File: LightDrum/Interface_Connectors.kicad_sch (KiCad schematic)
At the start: 6 parts, among them J6 0525593652, J7 0541323662, J8 PWR-CONN

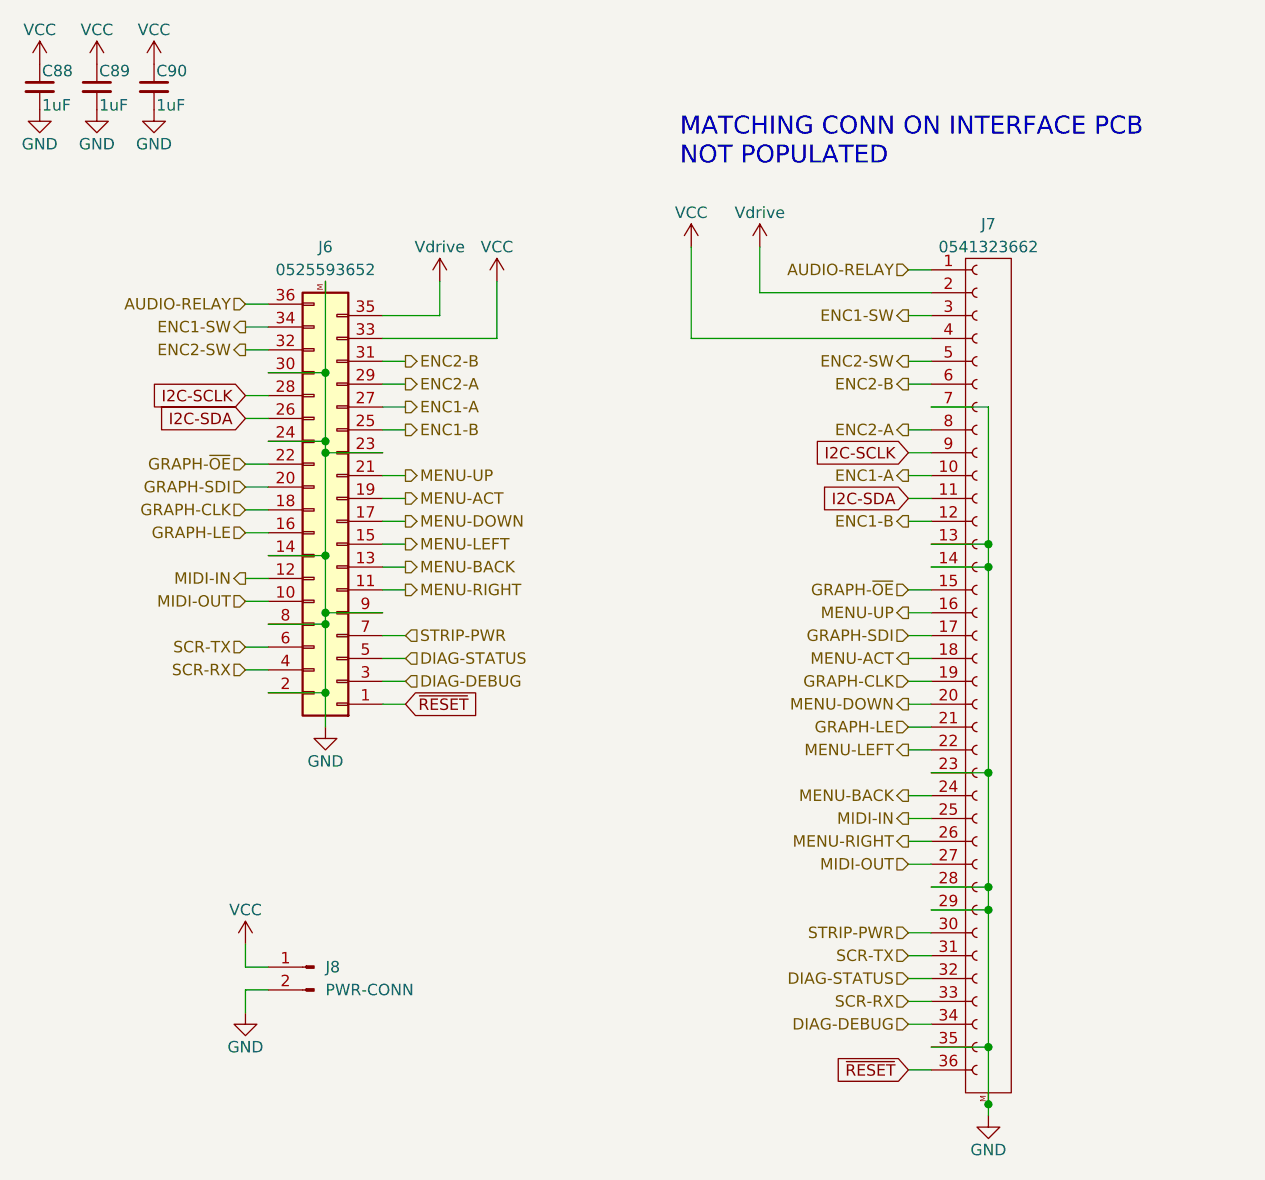
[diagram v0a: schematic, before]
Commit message: First pass over schematic (WIP)
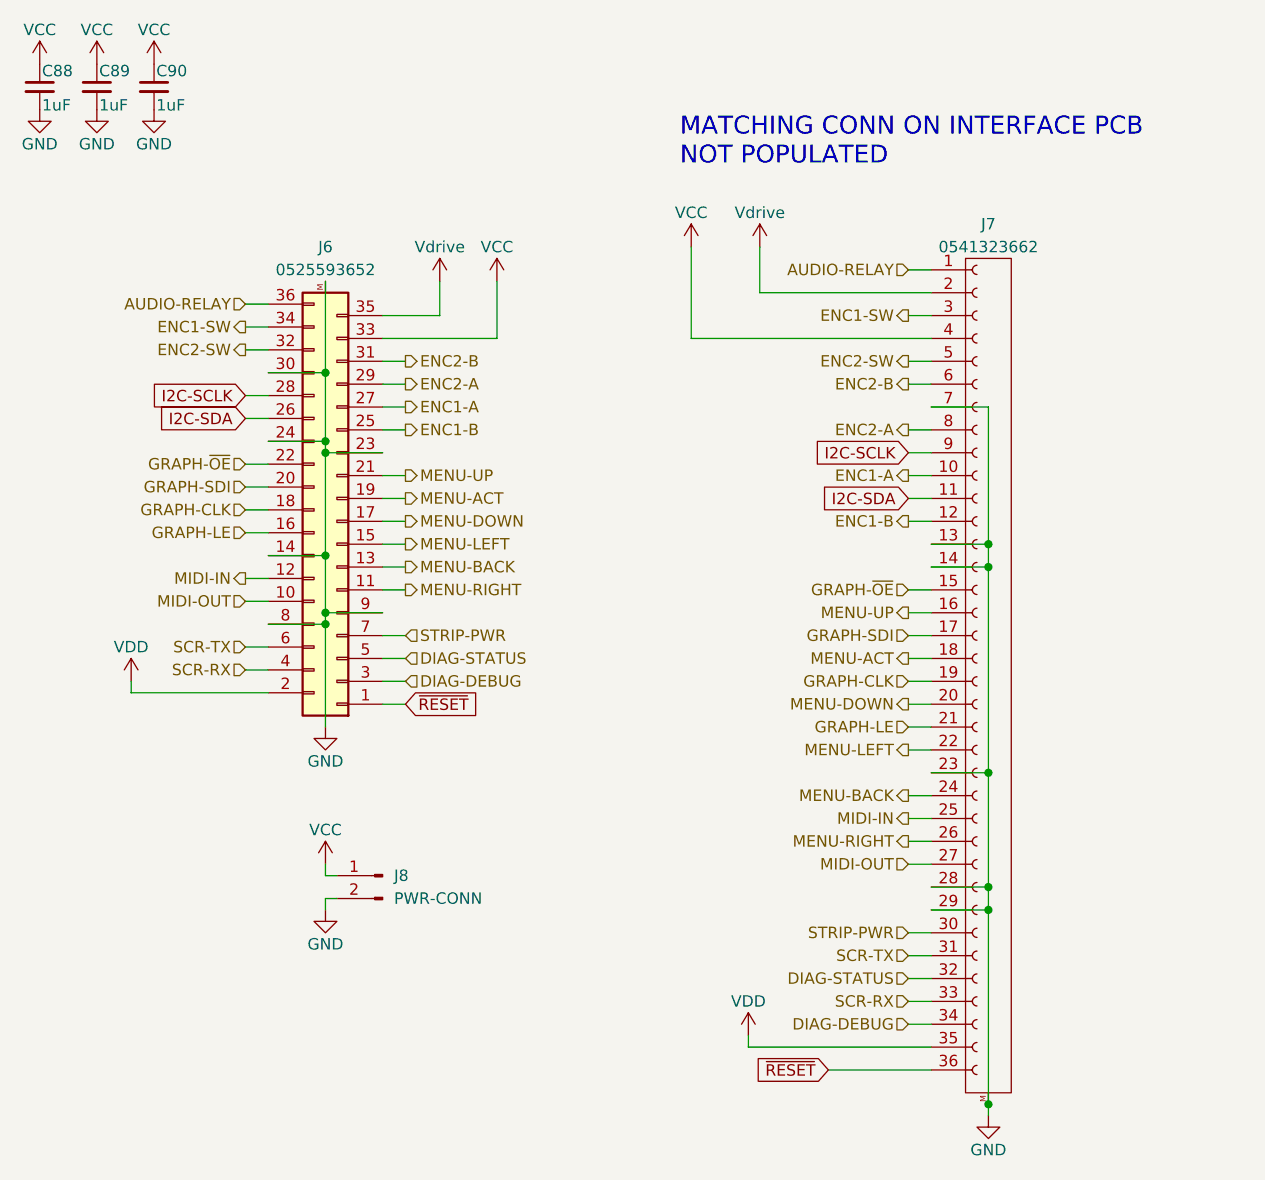
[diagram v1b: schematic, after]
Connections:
- net GND: no longer J6.2 (Pin_2), J7.35 (Pin_35)
- new net VDD: J6.2 (Pin_2), J7.35 (Pin_35)
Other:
- moved on the sheet: J8
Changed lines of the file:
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@@
   (title_block
     (title "LightDrum")
-    (rev "REV7")
+    (rev "REV8")
     (company "Daxxn Industries")
   )
-  (junction (at 50.8 90.17) (diameter 0) (color 0 0 0 0)
-  )
   (junction (at 124.46 76.2) (diameter 0) (color 0 0 0 0)
   )
@@
   (junction (at 50.8 62.23) (diameter 0) (color 0 0 0 0)
   )
-  (junction (at 124.46 129.54) (diameter 0) (color 0 0 0 0)
-  )
   (junction (at 50.8 54.61) (diameter 0) (color 0 0 0 0)
   )
@@
     (stroke (width 0) (type default) (color 0 0 0 0))
   )
-  (wire (pts (xy 44.45 120.65) (xy 41.91 120.65))
+  (wire (pts (xy 52.07 110.49) (xy 50.8 110.49))
     (stroke (width 0) (type default) (color 0 0 0 0))
   )
@@
     (stroke (width 0) (type default) (color 0 0 0 0))
   )
-  (wire (pts (xy 124.46 114.3) (xy 124.46 129.54))
-    (stroke (width 0) (type default) (color 0 0 0 0))
-  )
-  (wire (pts (xy 50.8 90.17) (xy 50.8 93.98))
+  (wire (pts (xy 124.46 114.3) (xy 124.46 135.89))
     (stroke (width 0) (type default) (color 0 0 0 0))
   )
@@
     (stroke (width 0) (type default) (color 0 0 0 0))
   )
-  (wire (pts (xy 115.57 132.08) (xy 118.11 132.08))
+  (wire (pts (xy 106.68 132.08) (xy 118.11 132.08))
     (stroke (width 0) (type default) (color 0 0 0 0))
   )
@@
     (stroke (width 0) (type default) (color 0 0 0 0))
   )
+  (wire (pts (xy 29.21 88.9) (xy 29.21 90.17))
+    (stroke (width 0) (type default) (color 0 0 0 0))
+  )
   (wire (pts (xy 91.44 40.64) (xy 91.44 50.8))
     (stroke (width 0) (type default) (color 0 0 0 0))
@@
     (stroke (width 0) (type default) (color 0 0 0 0))
   )
-  (wire (pts (xy 44.45 90.17) (xy 50.8 90.17))
-    (stroke (width 0) (type default) (color 0 0 0 0))
-  )
   (wire (pts (xy 69.85 50.8) (xy 57.15 50.8))
     (stroke (width 0) (type default) (color 0 0 0 0))
@@
     (stroke (width 0) (type default) (color 0 0 0 0))
   )
+  (wire (pts (xy 29.21 90.17) (xy 44.45 90.17))
+    (stroke (width 0) (type default) (color 0 0 0 0))
+  )
   (wire (pts (xy 118.11 121.92) (xy 115.57 121.92))
     (stroke (width 0) (type default) (color 0 0 0 0))
   )
-  (wire (pts (xy 50.8 82.55) (xy 50.8 90.17))
+  (wire (pts (xy 97.79 129.54) (xy 118.11 129.54))
+    (stroke (width 0) (type default) (color 0 0 0 0))
+  )
+  (wire (pts (xy 50.8 82.55) (xy 50.8 93.98))
     (stroke (width 0) (type default) (color 0 0 0 0))
   )
@@
     (stroke (width 0) (type default) (color 0 0 0 0))
   )
+  (wire (pts (xy 97.79 128.27) (xy 97.79 129.54))
+    (stroke (width 0) (type default) (color 0 0 0 0))
+  )
   (wire (pts (xy 91.44 50.8) (xy 118.11 50.8))
     (stroke (width 0) (type default) (color 0 0 0 0))
@@
     (stroke (width 0) (type default) (color 0 0 0 0))
   )
-  (wire (pts (xy 41.91 120.65) (xy 41.91 118.11))
+  (wire (pts (xy 50.8 110.49) (xy 50.8 109.22))
     (stroke (width 0) (type default) (color 0 0 0 0))
   )
@@
     (stroke (width 0) (type default) (color 0 0 0 0))
   )
-  (wire (pts (xy 118.11 129.54) (xy 124.46 129.54))
-    (stroke (width 0) (type default) (color 0 0 0 0))
-  )
   (wire (pts (xy 63.5 48.26) (xy 63.5 44.45))
     (stroke (width 0) (type default) (color 0 0 0 0))
@@
     (stroke (width 0) (type default) (color 0 0 0 0))
   )
-  (wire (pts (xy 44.45 123.19) (xy 41.91 123.19))
+  (wire (pts (xy 52.07 113.03) (xy 50.8 113.03))
     (stroke (width 0) (type default) (color 0 0 0 0))
   )
@@
     (stroke (width 0) (type default) (color 0 0 0 0))
   )
-  (wire (pts (xy 41.91 123.19) (xy 41.91 125.73))
+  (wire (pts (xy 50.8 113.03) (xy 50.8 114.3))
     (stroke (width 0) (type default) (color 0 0 0 0))
   )
@@
   )
   (wire (pts (xy 118.11 91.44) (xy 115.57 91.44))
-    (stroke (width 0) (type default) (color 0 0 0 0))
-  )
-  (wire (pts (xy 124.46 129.54) (xy 124.46 135.89))
     (stroke (width 0) (type default) (color 0 0 0 0))
   )
@@
     )
   )
-  (global_label "~{RESET}" (shape input) (at 115.57 132.08 180) (fields_autoplaced)
-    (effects (font (size 1.27 1.27)) (justify right))
-    (property "Intersheet References" "${INTERSHEET_REFS}" (id 0) (at 107.4117 132.0006 0)
+  (global_label "~{RESET}" (shape input) (at 106.68 132.08 180) (fields_autoplaced)
+    (effects (font (size 1.27 1.27)) (justify right))
+    (property "Intersheet References" "${INTERSHEET_REFS}" (id 0) (at 98.5217 132.0006 0)
       (effects (font (size 1.27 1.27)) (justify right) hide)
     )
@@
     (pin "1")
   )
-  (symbol (lib_id "power:GND") (at 41.91 125.73 0) (unit 1)
-    (in_bom yes) (on_board yes)
-    (property "Reference" "#PWR0135" (id 0) (at 41.91 132.08 0)
-      (effects (font (size 1.27 1.27)) hide)
-    )
-    (property "Value" "GND" (id 1) (at 41.91 129.54 0))
-    (property "Footprint" "" (id 2) (at 41.91 125.73 0)
-      (effects (font (size 1.27 1.27)) hide)
-    )
-    (property "Datasheet" "" (id 3) (at 41.91 125.73 0)
+  (symbol (lib_id "power:GND") (at 50.8 114.3 0) (unit 1)
+    (in_bom yes) (on_board yes)
+    (property "Reference" "#PWR0135" (id 0) (at 50.8 120.65 0)
+      (effects (font (size 1.27 1.27)) hide)
+    )
+    (property "Value" "GND" (id 1) (at 50.8 118.11 0))
+    (property "Footprint" "" (id 2) (at 50.8 114.3 0)
+      (effects (font (size 1.27 1.27)) hide)
+    )
+    (property "Datasheet" "" (id 3) (at 50.8 114.3 0)
       (effects (font (size 1.27 1.27)) hide)
     )
@@
     (pin "1")
   )
+  (symbol (lib_id "power:VDD") (at 97.79 128.27 0) (unit 1)
+    (in_bom yes) (on_board yes)
+    (property "Reference" "#PWR069" (id 0) (at 97.79 132.08 0)
+      (effects (font (size 1.27 1.27)) hide)
+    )
+    (property "Value" "VDD" (id 1) (at 97.79 124.46 0))
+    (property "Footprint" "" (id 2) (at 97.79 128.27 0)
+      (effects (font (size 1.27 1.27)) hide)
+    )
+    (property "Datasheet" "" (id 3) (at 97.79 128.27 0)
+      (effects (font (size 1.27 1.27)) hide)
+    )
+    (pin "1")
+  )
   (symbol (lib_id "power:Vdrive") (at 63.5 44.45 0) (unit 1)
     (in_bom yes) (on_board yes)
@@
     (pin "1")
   )
-  (symbol (lib_id "Connector:Conn_01x02_Male") (at 49.53 120.65 0) (mirror y) (unit 1)
-    (in_bom yes) (on_board yes)
-    (property "Reference" "J8" (id 0) (at 50.8 120.65 0)
+  (symbol (lib_id "Connector:Conn_01x02_Male") (at 57.15 110.49 0) (mirror y) (unit 1)
+    (in_bom yes) (on_board yes)
+    (property "Reference" "J8" (id 0) (at 58.42 110.49 0)
       (effects (font (size 1.27 1.27)) (justify right))
     )
-    (property "Value" "PWR-CONN" (id 1) (at 50.8 123.19 0)
+    (property "Value" "PWR-CONN" (id 1) (at 58.42 113.03 0)
       (effects (font (size 1.27 1.27)) (justify right))
     )
-    (property "Footprint" "Connector_JST:JST_XA_B02B-XASK-1_1x02_P2.50mm_Vertical" (id 2) (at 49.53 120.65 0)
-      (effects (font (size 1.27 1.27)) hide)
-    )
-    (property "Datasheet" "~" (id 3) (at 49.53 120.65 0)
+    (property "Footprint" "Connector_JST:JST_XA_B02B-XASK-1_1x02_P2.50mm_Vertical" (id 2) (at 57.15 110.49 0)
+      (effects (font (size 1.27 1.27)) hide)
+    )
+    (property "Datasheet" "~" (id 3) (at 57.15 110.49 0)
       (effects (font (size 1.27 1.27)) hide)
     )
     (pin "1")
     (pin "2")
+  )
+  (symbol (lib_id "power:VDD") (at 29.21 88.9 0) (unit 1)
+    (in_bom yes) (on_board yes)
+    (property "Reference" "#PWR068" (id 0) (at 29.21 92.71 0)
+      (effects (font (size 1.27 1.27)) hide)
+    )
+    (property "Value" "VDD" (id 1) (at 29.21 85.09 0))
+    (property "Footprint" "" (id 2) (at 29.21 88.9 0)
+      (effects (font (size 1.27 1.27)) hide)
+    )
+    (property "Datasheet" "" (id 3) (at 29.21 88.9 0)
+      (effects (font (size 1.27 1.27)) hide)
+    )
+    (pin "1")
   )
   (symbol (lib_id "power:GND") (at 19.05 25.4 0) (unit 1)
@@
     (pin "1")
   )
-  (symbol (lib_id "power:VCC") (at 41.91 118.11 0) (unit 1)
-    (in_bom yes) (on_board yes)
-    (property "Reference" "#PWR0136" (id 0) (at 41.91 121.92 0)
-      (effects (font (size 1.27 1.27)) hide)
-    )
-    (property "Value" "VCC" (id 1) (at 41.91 114.3 0))
-    (property "Footprint" "" (id 2) (at 41.91 118.11 0)
-      (effects (font (size 1.27 1.27)) hide)
-    )
-    (property "Datasheet" "" (id 3) (at 41.91 118.11 0)
-      (effects (font (size 1.27 1.27)) hide)
-    )
+  (symbol (lib_id "power:VCC") (at 50.8 109.22 0) (unit 1)
+    (in_bom yes) (on_board yes)
+    (property "Reference" "#PWR0136" (id 0) (at 50.8 113.03 0)
+      (effects (font (size 1.27 1.27)) hide)
+    )
+    (property "Value" "VCC" (id 1) (at 50.8 105.41 0))
+    (property "Footprint" "" (id 2) (at 50.8 109.22 0)
+      (effects (font (size 1.27 1.27)) hide)
+    )
+    (property "Datasheet" "" (id 3) (at 50.8 109.22 0)
+      (effects (font (size 1.27 1.27)) hide)
+    )
